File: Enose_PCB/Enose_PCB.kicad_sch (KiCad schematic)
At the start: 53 parts, among them IC3 TPS22958DGNR, J1 Conn_01x04_Pin, J10 Fan, J11 Conn_01x04_Pin, J2 Conn_01x04_Pin, J3 Conn_01x04_Pin, J4 DA15_Pins, Q6 NMOS, SW1 SW_SPST, SW2 SW_SPST, SW4 SW_SPDT, U1 ESP32-S3-WROOM-1

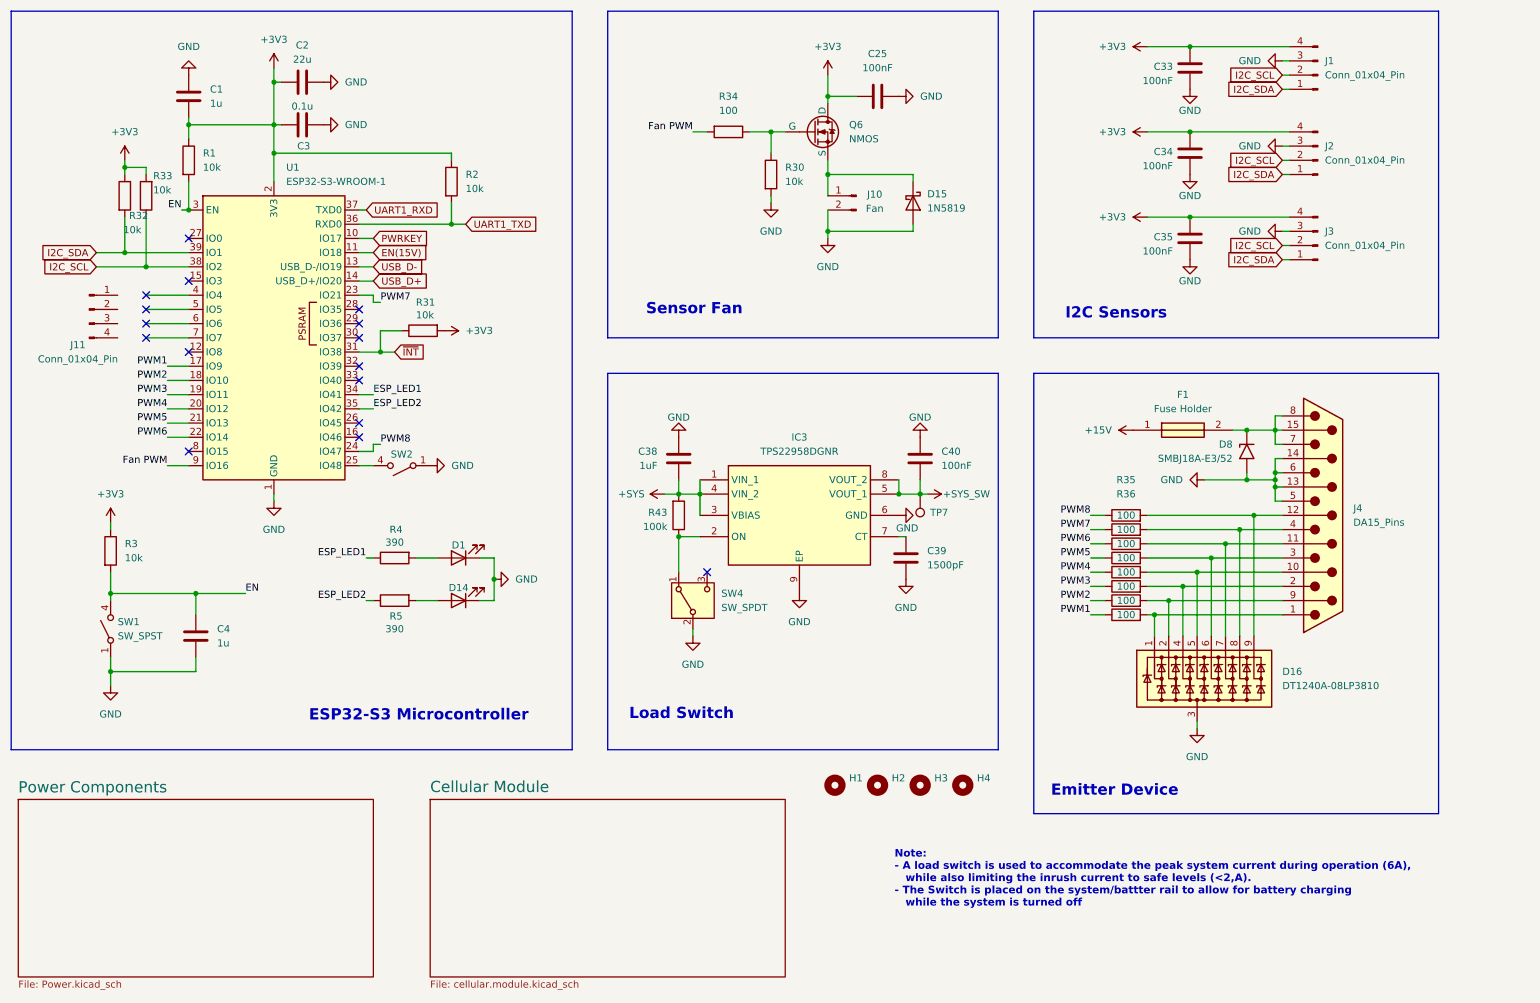
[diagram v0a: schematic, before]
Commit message: Enose PCB almost done
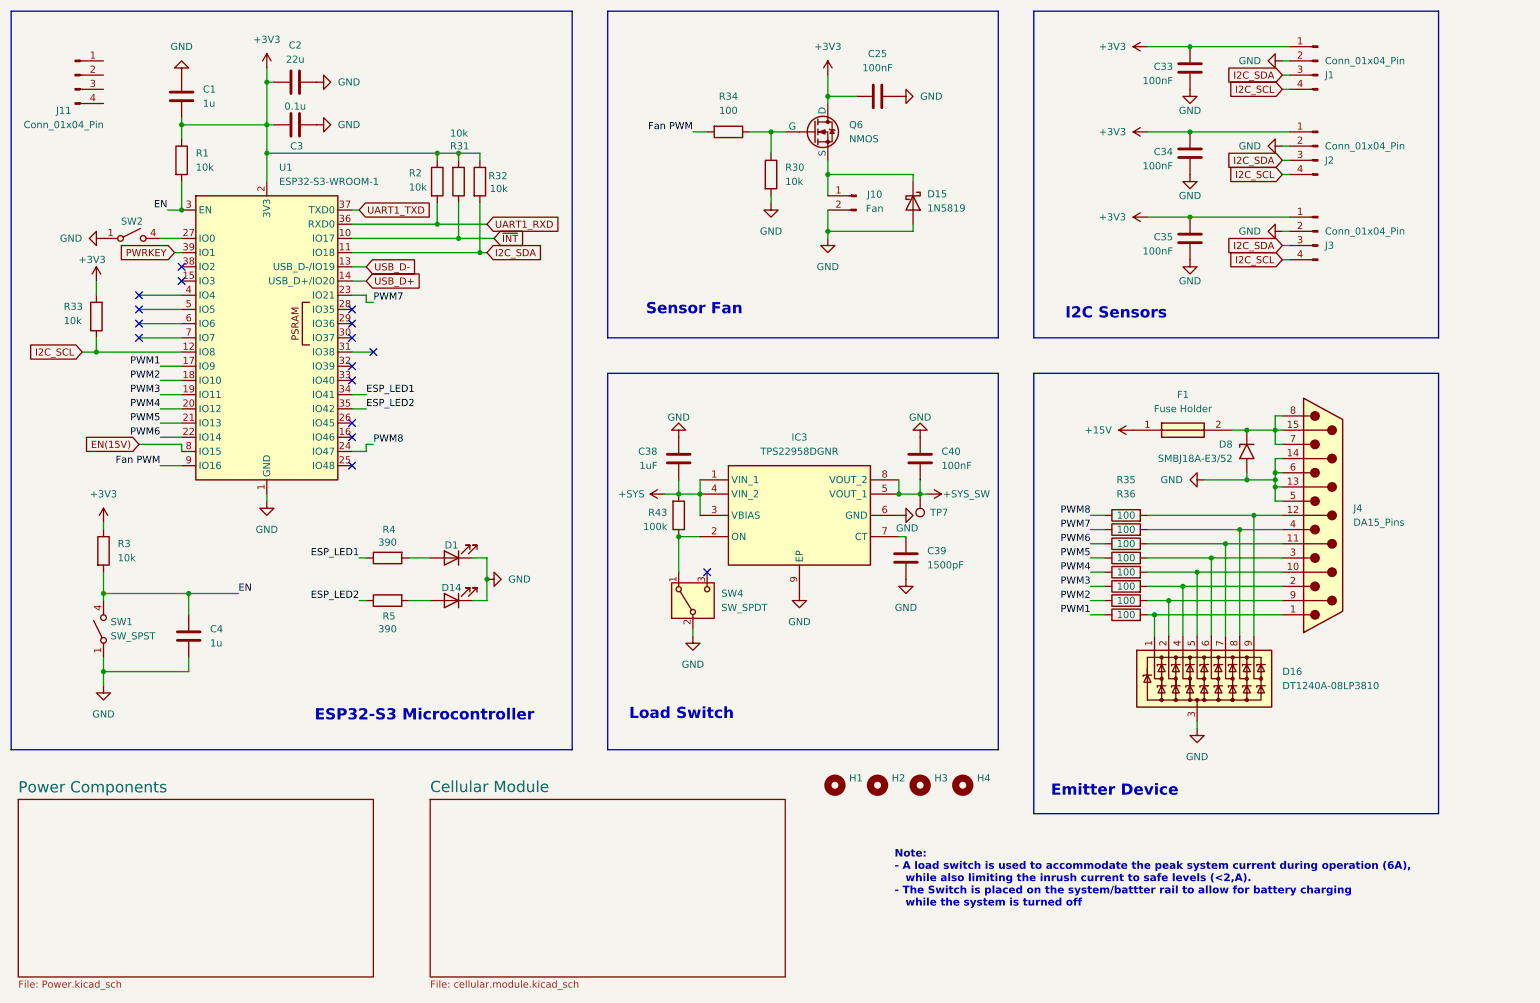
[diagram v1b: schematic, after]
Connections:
- net +3V3: now also J1.1 (Pin_1), J2.1 (Pin_1), J3.1 (Pin_1); no longer J1.4 (Pin_4), J2.4 (Pin_4), J3.4 (Pin_4)
- net EN(15V): now also U1.8 (IO15); no longer U1.11 (IO18)
- net GND: now also J1.2 (Pin_2), J2.2 (Pin_2), J3.2 (Pin_2); no longer J1.3 (Pin_3), J2.3 (Pin_3), J3.3 (Pin_3)
- net I2C_SCL: now also J1.4 (Pin_4), J2.4 (Pin_4), J3.4 (Pin_4), U1.12 (IO8); no longer J1.2 (Pin_2), J2.2 (Pin_2), J3.2 (Pin_2), U1.38 (IO2)
- net I2C_SDA: now also J1.3 (Pin_3), J2.3 (Pin_3), J3.3 (Pin_3), U1.11 (IO18); no longer J1.1 (Pin_1), J2.1 (Pin_1), J3.1 (Pin_1), U1.39 (IO1)
- net PWRKEY: now also U1.39 (IO1); no longer U1.10 (IO17)
- net UART1_RXD: now also R2.2, U1.36 (RXD0); no longer U1.37 (TXD0)
- net UART1_TXD: now also U1.37 (TXD0); no longer R2.2, U1.36 (RXD0)
- net ~{INT}: now also U1.10 (IO17); no longer U1.31 (IO38)
- net at U1.25 (IO48): no longer SW2.4 (B)
- net at U1.27 (IO0): now also SW2.4 (B)
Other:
- moved on the sheet: C1, C2, C3, C4, D1, D14, J1, J11, J2, J3, R1, R2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
